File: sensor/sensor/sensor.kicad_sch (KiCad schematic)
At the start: 34 parts, among them J1 RJ12_Shielded, J2 Conn_01x04, J3 Conn_01x06, SW1 SW_SPST, SW2 SW_SPST, SW3 SW_SPST, SW4 SW_SPST, U1 PCA9615DP, U2 LTC4316xDD, U5 TPS73101DBV

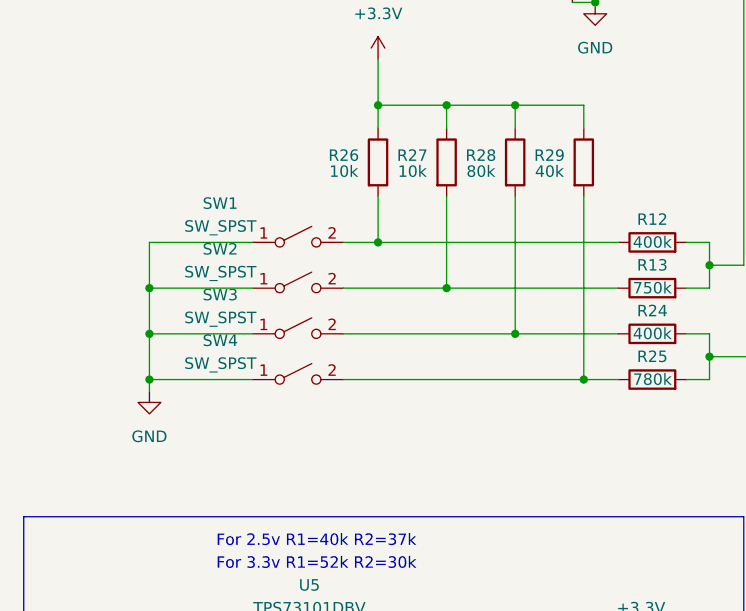
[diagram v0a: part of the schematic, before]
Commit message: half way done with board
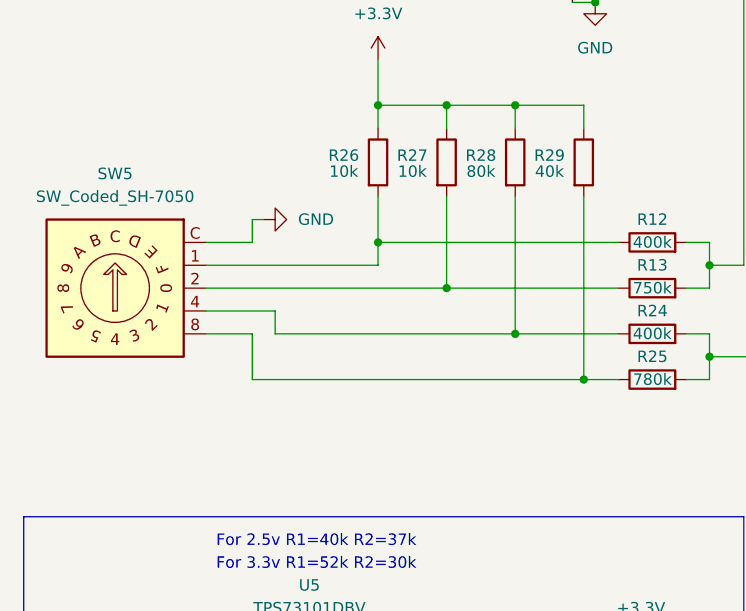
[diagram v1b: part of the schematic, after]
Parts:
- removed SW1, SW2, SW3, SW4: SW_SPST, symbol Switch:SW_SPST
- added SW5: SW_Coded_SH-7050, RJ12_Pin_Connector:Rotary_Switch_16_pos, symbol Switch:SW_Coded_SH-7050
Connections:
- net GND: now also SW5.C
- net at R13.1, R27.2: now also SW5.2
- net at R12.1, R26.2: now also SW5.1
- net at R25.1, R29.2: now also SW5.8
- net at R24.1, R28.2: now also SW5.4
